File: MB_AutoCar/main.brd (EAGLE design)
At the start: 213.4 x 108 mm, 48 parts, among them J2 Out1, J4 Out2, K1 CQ1-12V, K2 CQ1-12V, K3 CQ1-12V, K4 CQ1-12V, Q1 PN2222, Q2 PN2222, Q3 PN2222, Q4 PN2222, U1 ARDUINO-MEGAFULL

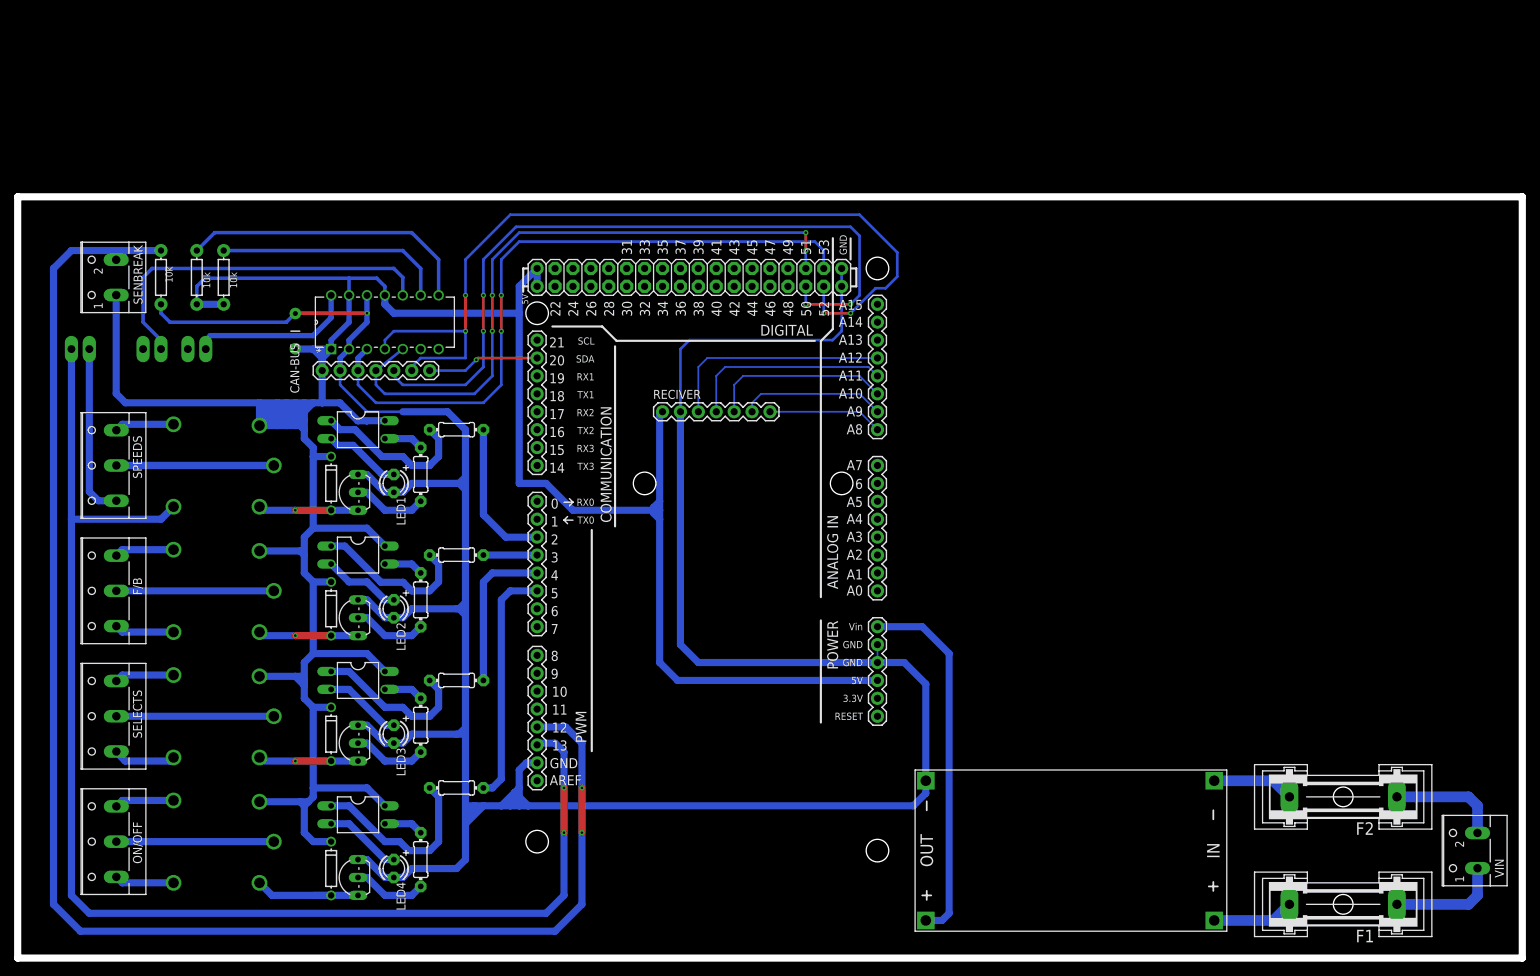
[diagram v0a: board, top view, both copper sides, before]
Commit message: update
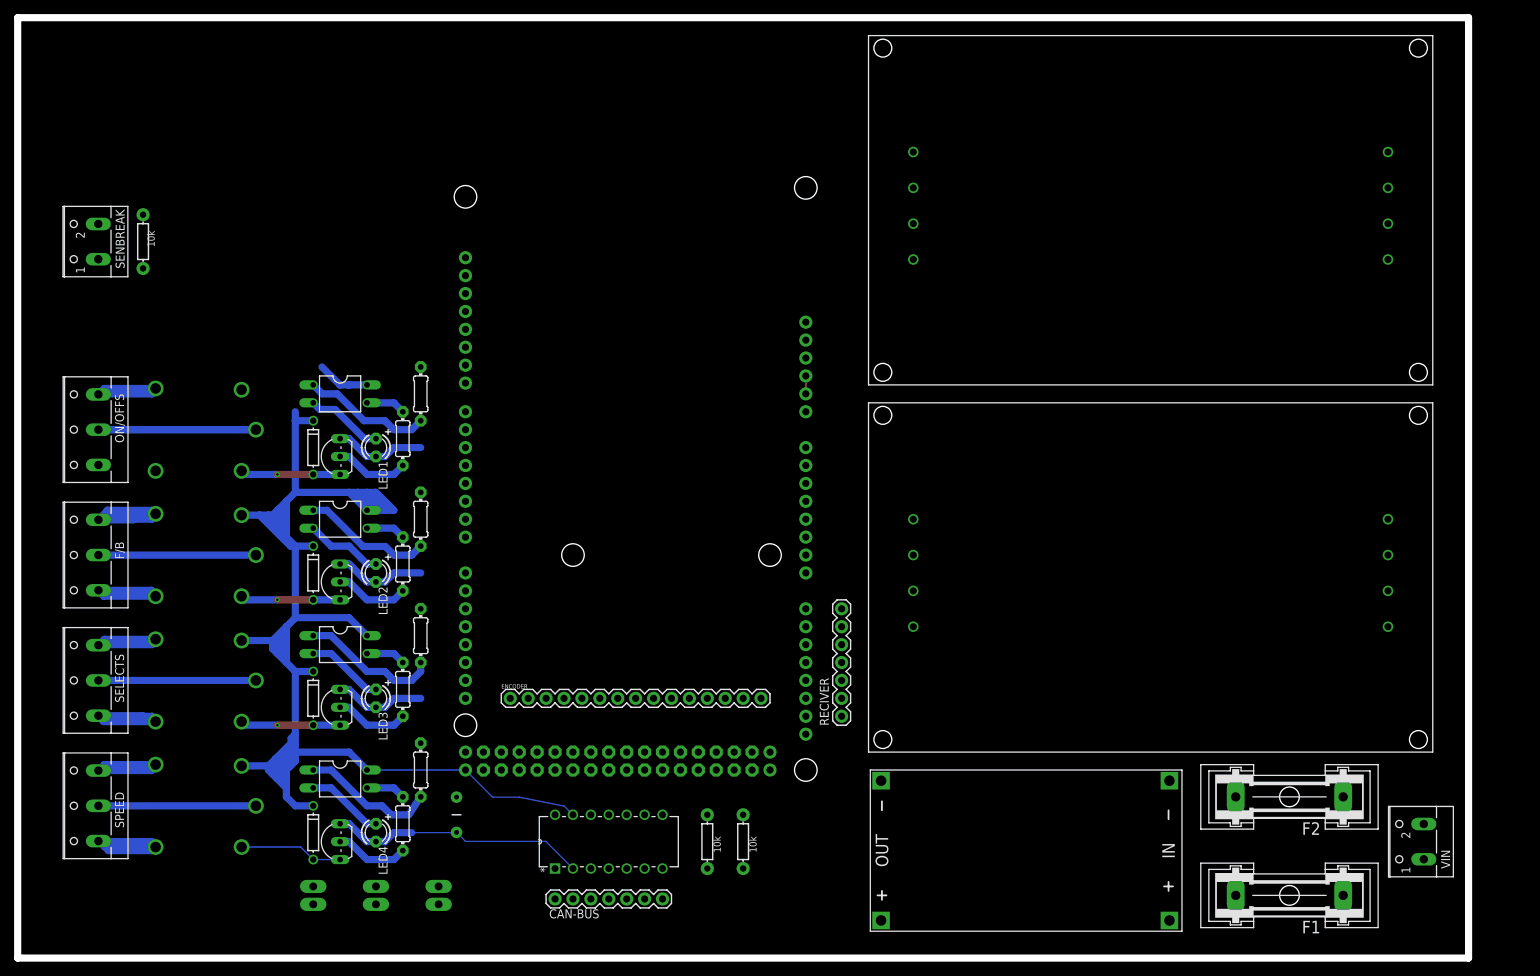
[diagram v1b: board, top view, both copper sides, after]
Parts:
- removed ON/OFF, SPEEDS: (no value), con-wago-500:W237-103
- removed PWMS: Out1, SparkFun-Connectors:1X02_LONGPADS
- added ENCODER: (no value), SparkFun-Connectors:1X15
- added ON/OFFS, SPEED: (no value), con-wago-500:W237-103
- added PWMS1: Out1, SparkFun-Connectors:1X02_LONGPADS
- added U$3, U$4: (no value), TLP250:TLP250
- moved U1 122.3 mm to (114.3, 123.2), flipped to the bottom, turned to 270 degrees
- moved R13 111.4 mm to (102.9, 16.5)
- moved R12 105.4 mm to (97.8, 16.5)
- moved J4 88.0 mm to (59.7, 7.62), turned to 90 degrees
- moved J2 82.4 mm to (50.8, 7.62), turned to 90 degrees
- moved CAN-BUS 81.9 mm to (76.2, 8.38)
- moved U$1 80.2 mm to (91.4, 20.3)
- moved C2 72.3 mm to (62.2, 20.3), turned to 90 degrees
- moved RECIVER 50.1 mm to (116.8, 34.3), turned to 90 degrees
- moved R1 8.13 mm to (57.1, 45.7), turned to 270 degrees
- moved VIN 7.73 mm to (198.1, 16.5)
- moved F1 7.73 mm to (180.3, 8.89)
- moved F2 7.62 mm to (180.3, 22.9)
- moved R3 7.18 mm to (57.1, 62.2), turned to 270 degrees
- moved R7 7.18 mm to (57.1, 80.0), turned to 270 degrees
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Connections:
- removed net N$13: K4.NO, ON/OFF.1
- removed net PWMS: PWMS.1, SPEEDS.1
- new net D22: ENCODER.1, U1.22
- new net D24: ENCODER.2, U1.24
- new net D26: ENCODER.3, U1.26
- new net D28: ENCODER.4, U1.28
- new net D30: ENCODER.5, U1.30
- new net D32: ENCODER.6, U1.32
- new net D34: ENCODER.7, U1.34
- new net D36: ENCODER.8, U1.36
- new net D38: ENCODER.9, U1.38
- new net D40: ENCODER.10, U1.40
- new net D42: ENCODER.11, U1.42
- new net D44: ENCODER.12, U1.44
- new net D46: ENCODER.13, U1.46
- new net N$1: PWMS1.1, SPEED.1
- new net N$2: K1.NO, ON/OFFS.1
- new net VIN: ENCODER.14
- net D12PWM: now also K4.NO, PWMS1.2
- net D13PWM: no longer K1.NO, PWMS.2
- net GND: now also ENCODER.15
- net IN1: now also U1.5; no longer U1.2
- net IN2: now also U1.4; no longer U1.3
- net IN3: now also U1.3; no longer U1.4
- net IN4: now also U1.2; no longer U1.5
- net N$14: now also SPEED.2; no longer ON/OFF.2
- net N$15: now also ON/OFFS.3; no longer SPEEDS.3
- net N$18: now also SPEED.3; no longer ON/OFF.3
- net N$3: now also ON/OFFS.2; no longer SPEEDS.2
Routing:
- net GND: track 435.4 -> 78.3 mm, vias 2 -> 0
- net VCC: track 447.4 -> 237.8 mm
- net D12PWM: track 217.8 -> 24.1 mm, vias 2 -> 0
- net D13PWM: track 189.5 -> 0.00 mm, vias 2 -> 0
- net SCK: track 121.7 -> 0.00 mm, vias 4 -> 0
- net MISO: track 105.2 -> 0.00 mm, vias 4 -> 0
- net !CS: track 95.6 -> 0.00 mm, vias 2 -> 0
- net MOSI: track 92.6 -> 0.00 mm, vias 4 -> 0
- net VINS: track 52.3 -> 0.00 mm
- net N$21: track 51.6 -> 0.00 mm
- net D7: track 42.0 -> 0.00 mm
- net IN4: track 34.1 -> 0.00 mm
- net !SHDN: track 32.8 -> 0.00 mm
- net A12: track 32.3 -> 0.00 mm
- net A11: track 29.0 -> 0.00 mm
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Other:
- board size 213.4 x 108 mm -> 205.7 x 133.3 mm
